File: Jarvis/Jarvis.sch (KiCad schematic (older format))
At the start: 143 parts, among them IC1 ADP1607, IC2 MAX-8Q, IC3 MPU-9250, IC4 STM32F411CxUx, IC5 Si4460, IC6 MS5611-01BA03, J1 PYRO, J2 PWR, J3 ARM, P1 SMA, P2 SMA, P3 SWD_TC, Q1 PFET, Q2 PFET, Q3 PFET, Q4 NFET, Q5 NFET, Q6 NFET, Q7 NFET, U1 MICROSD, X1 434MHz ANT, X10 Housing x1, X11 Housing x3, X12 M Crimps x6, X13 F Crimps x17, X14 Crimp Tool, X2 Red LED, X3 AA Battery, X4 AA Holder, X5 ARM Switch, X6 Wire, X7 Heat Shrink, X8 Housing x1, X9 Housing x4, Y1 26MHz, Y2 30MHz

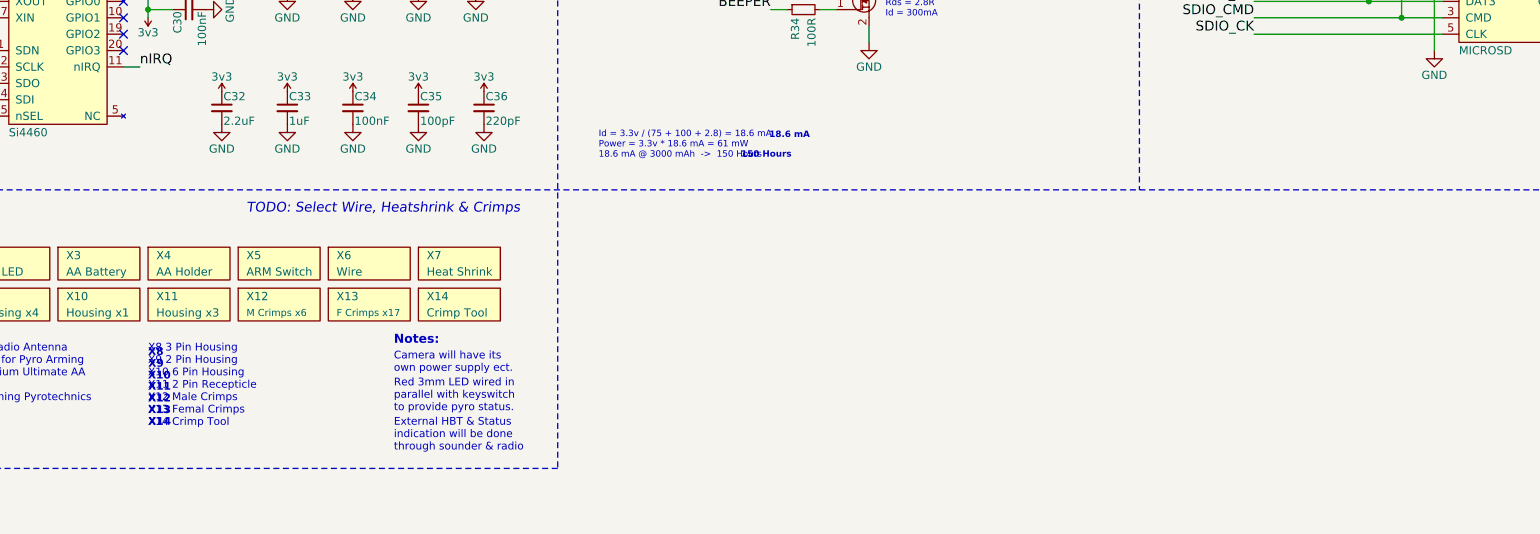
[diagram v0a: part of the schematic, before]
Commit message: Added Testpoints
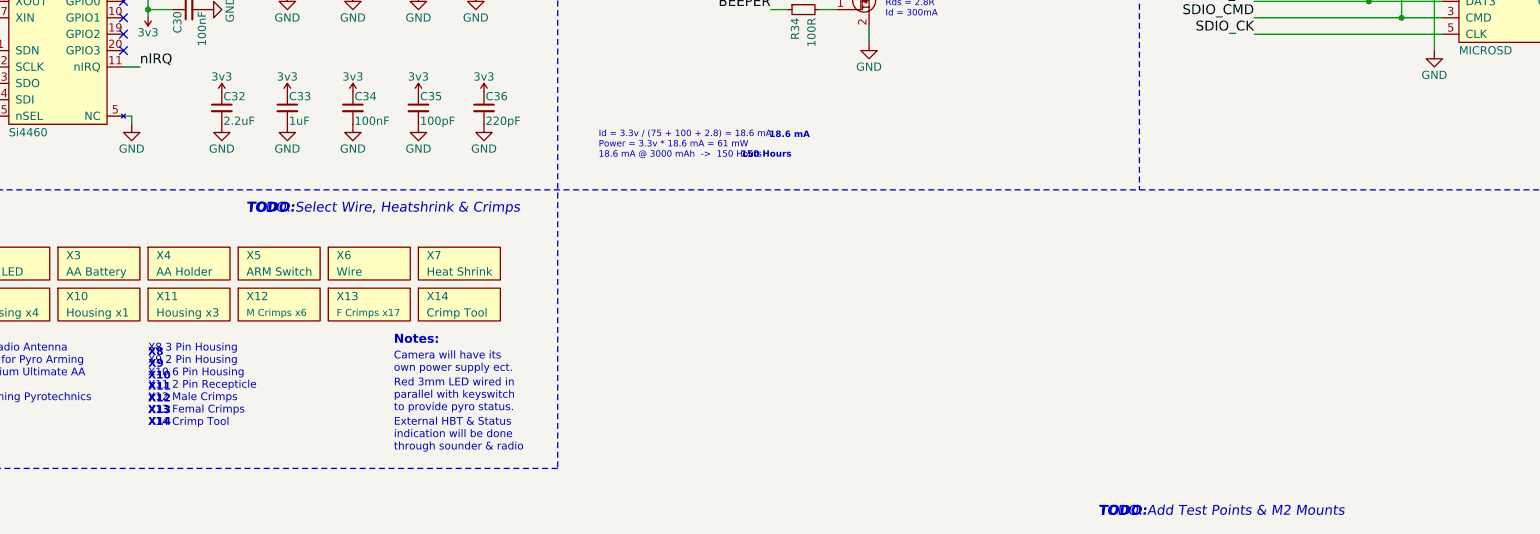
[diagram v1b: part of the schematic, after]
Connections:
- net GND: now also IC5.5 (NC)
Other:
- note added: "TODO:"
- note added: "TODO: Add Test Points & M2 Mounts"
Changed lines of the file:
@@
 Text Notes 6650 8250 0    60   Italic 0
 TODO: Select Wire, Heatshrink & Crimps
+Wire Wire Line
+	5900 7650 5950 7650
+Wire Wire Line
+	5950 7650 5950 7700
+$Comp
+L GND #PWR?
+U 1 1 56FD5801
+P 5950 7700
+F 0 "#PWR?" H 5950 7450 50  0001 C CNN
+F 1 "GND" H 5950 7550 50  0000 C CNN
+F 2 "" H 5950 7700 50  0000 C CNN
+F 3 "" H 5950 7700 50  0000 C CNN
+	1    5950 7700
+	1    0    0    -1
+$EndComp
+Text Notes 11850 10100 0    60   Italic 0
+TODO: Add Test Points & M2 Mounts
+Text Notes 11850 10100 0    60   Italic 12
+TODO:
+Text Notes 6650 8250 0    60   Italic 12
+TODO:
 $EndSCHEMATC

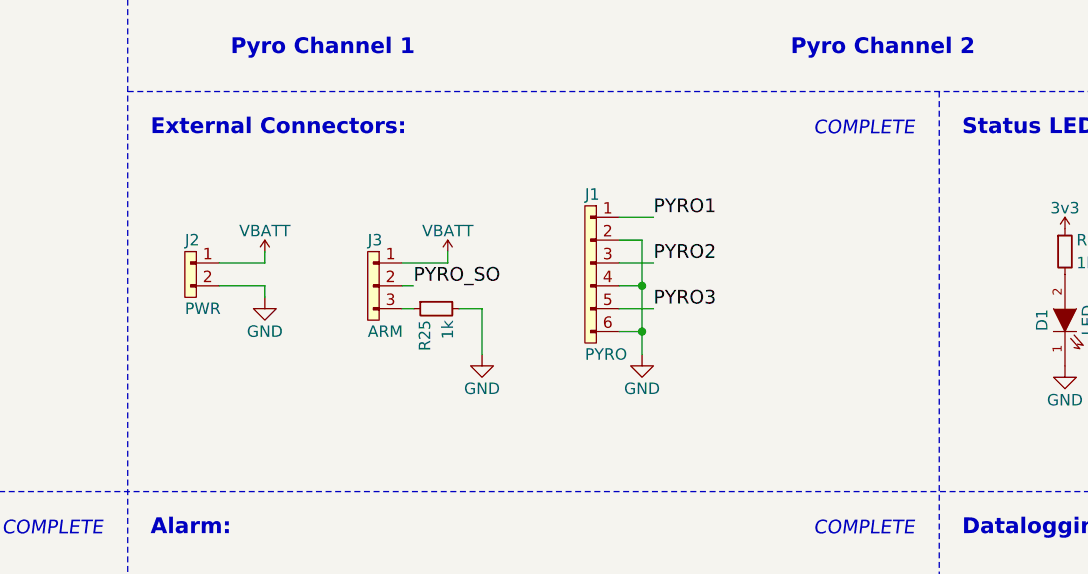
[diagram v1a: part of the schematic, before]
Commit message: Started PCB layout
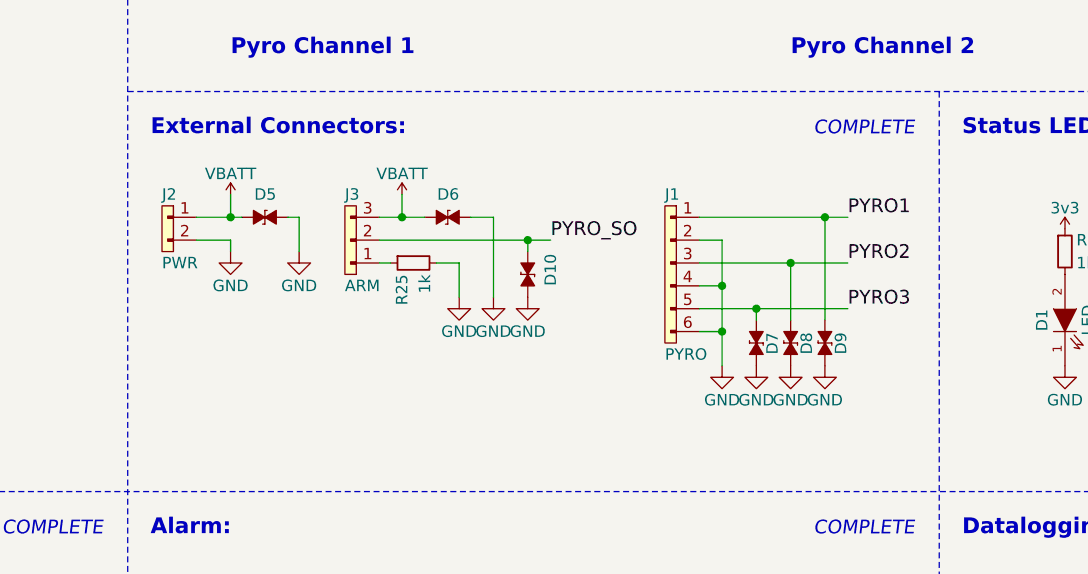
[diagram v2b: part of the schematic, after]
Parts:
- added D10, D5, D6, D7, D8, D9: ESD_DIODE, agg:0402-L, symbol ESD_DIODE
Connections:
- net GND: now also D10.1, D5.1, D6.1, D7.1, D8.1, D9.1
- net PYRO1: now also D9.2
- net PYRO2: now also D8.2
- net PYRO3: now also D7.2
- net PYRO_SO: now also D10.2
- net VBATT: now also J3.3, D5.2, D6.2; no longer J3.1
- net at R25.1: now also J3.1; no longer J3.3
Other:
- moved on the sheet: J1, J2, J3, R25
